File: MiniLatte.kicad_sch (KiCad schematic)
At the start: 23 parts, among them CN5 WAFER-PH2.0-4PZZ, CN6 47053-1000, CN8 SMTWE2055MTJ, CN9 SMTWE2055MTJ, SW6 DSHP01TSGER, U19 TPS54202DDCR, U22 W25N01GVZEIG_C907680

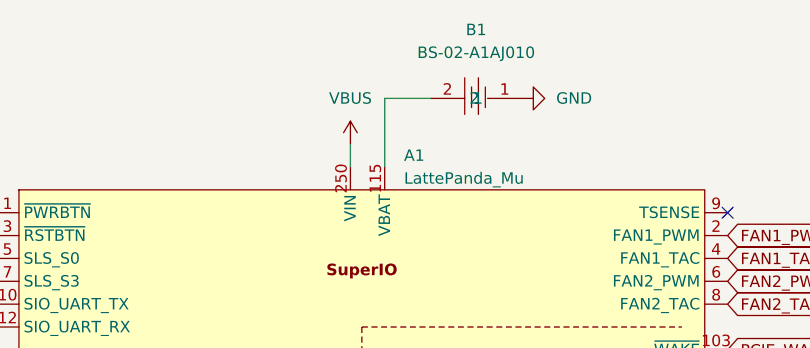
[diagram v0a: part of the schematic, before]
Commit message: .
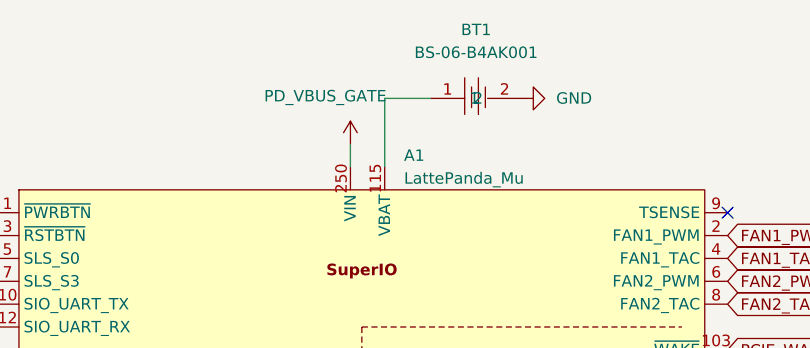
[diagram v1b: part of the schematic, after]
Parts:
- removed B1: BS-02-A1AJ010, easyeda2kicad:BAT-TH_BS-02-A1AJ010, symbol da:BS-02-A1AJ010
- added BT1: BS-06-B4AK001, easyeda2kicad:BAT-SMD_BS-06-B4AA012, symbol da:BS-06-B4AK001
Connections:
- net VBUS is gone; now on net PD_VBUS_GATE: A1.250 (VIN), A1.251 (VIN), A1.252 (VIN), A1.253 (VIN), A1.254 (VIN), A1.255 (VIN), A1.256 (VIN), A1.257 (VIN), A1.258 (VIN), A1.259 (VIN), A1.260 (VIN)
- net GND: now also BT1.2
- net at A1.115 (VBAT): now also BT1.1
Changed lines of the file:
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@@
-	)
-	(symbol
-		(lib_id "da:BS-02-A1AJ010")
-		(at 148.59 25.4 180)
-		(unit 1)
-		(exclude_from_sim no)
-		(in_bom yes)
-		(on_board yes)
-		(dnp no)
-		(fields_autoplaced yes)
-		(property "Reference" "B1"
-			(at 148.59 17.78 0)
-			(effects
-				(font
-					(size 1.27 1.27)
-				)
-			)
-		)
-		(property "Value" "BS-02-A1AJ010"
-			(at 148.59 20.32 0)
-			(effects
-				(font
-					(size 1.27 1.27)
-				)
-			)
-		)
-		(property "Footprint" "easyeda2kicad:BAT-TH_BS-02-A1AJ010"
-			(at 148.59 17.78 0)
-			(effects
-				(font
-					(size 1.27 1.27)
-				)
-				(hide yes)
-			)
-		)
-		(property "Datasheet" ""
-			(at 148.59 25.4 0)
-			(effects
-				(font
-					(size 1.27 1.27)
-				)
-				(hide yes)
-			)
-		)
-		(property "Description" ""
-			(at 148.59 25.4 0)
-			(effects
-				(font
-					(size 1.27 1.27)
-				)
-				(hide yes)
-			)
-		)
-		(property "LCSC Part" "C5239862"
-			(at 148.59 15.24 0)
-			(effects
-				(font
-					(size 1.27 1.27)
-				)
-				(hide yes)
-			)
-		)
-		(pin "1"
-		)
-		(pin "2"
-		)
-		(instances
-			(project ""
-				(path "/ffe475c5-d6e9-41b5-8ca1-322659dd88d8"
-					(reference "B1")
-					(unit 1)
-				)
-			)
-		)
 	)
 	(symbol
@@
 		(on_board yes)
 		(dnp no)
-		(fields_autoplaced yes)
 		(property "Reference" "#PWR04"
 			(at 134.62 34.29 0)
@@
 			)
 		)
-		(property "Value" "VBUS"
-			(at 134.62 25.4 0)
+		(property "Value" "PD_VBUS_GATE"
+			(at 131.826 25.146 0)
 			(effects
 				(font
@@
 					(unit 1)
 				)
+			)
+		)
+	)
+	(symbol
+		(lib_id "da:BS-06-B4AK001")
+		(at 148.59 25.4 0)
+		(unit 1)
+		(exclude_from_sim no)
+		(in_bom yes)
+		(on_board yes)
+		(dnp no)
+		(fields_autoplaced yes)
+		(property "Reference" "BT1"
+			(at 148.59 17.78 0)
+			(effects
+				(font
+					(size 1.27 1.27)
+				)
+			)
+		)
+		(property "Value" "BS-06-B4AK001"
+			(at 148.59 20.32 0)
+			(effects
+				(font
+					(size 1.27 1.27)
+				)
+			)
+		)
+		(property "Footprint" "easyeda2kicad:BAT-SMD_BS-06-B4AA012"
+			(at 148.59 33.02 0)
+			(effects
+				(font
+					(size 1.27 1.27)
+				)
+				(hide yes)
+			)
+		)
+		(property "Datasheet" ""
+			(at 148.59 25.4 0)
+			(effects
+				(font
+					(size 1.27 1.27)
+				)
+				(hide yes)
+			)
+		)
+		(property "Description" ""
+			(at 148.59 25.4 0)
+			(effects
+				(font
+					(size 1.27 1.27)
+				)
+				(hide yes)
+			)
+		)
+		(property "LCSC Part" "C964760"
+			(at 148.59 35.56 0)
+			(effects
+				(font
+					(size 1.27 1.27)
+				)
+				(hide yes)
+			)
+		)
+		(pin "2"
+		)
+		(pin "1"
+		)
+		(instances
+			(project ""
+				(path "/ffe475c5-d6e9-41b5-8ca1-322659dd88d8"
+					(reference "BT1")
+					(unit 1)
+				)

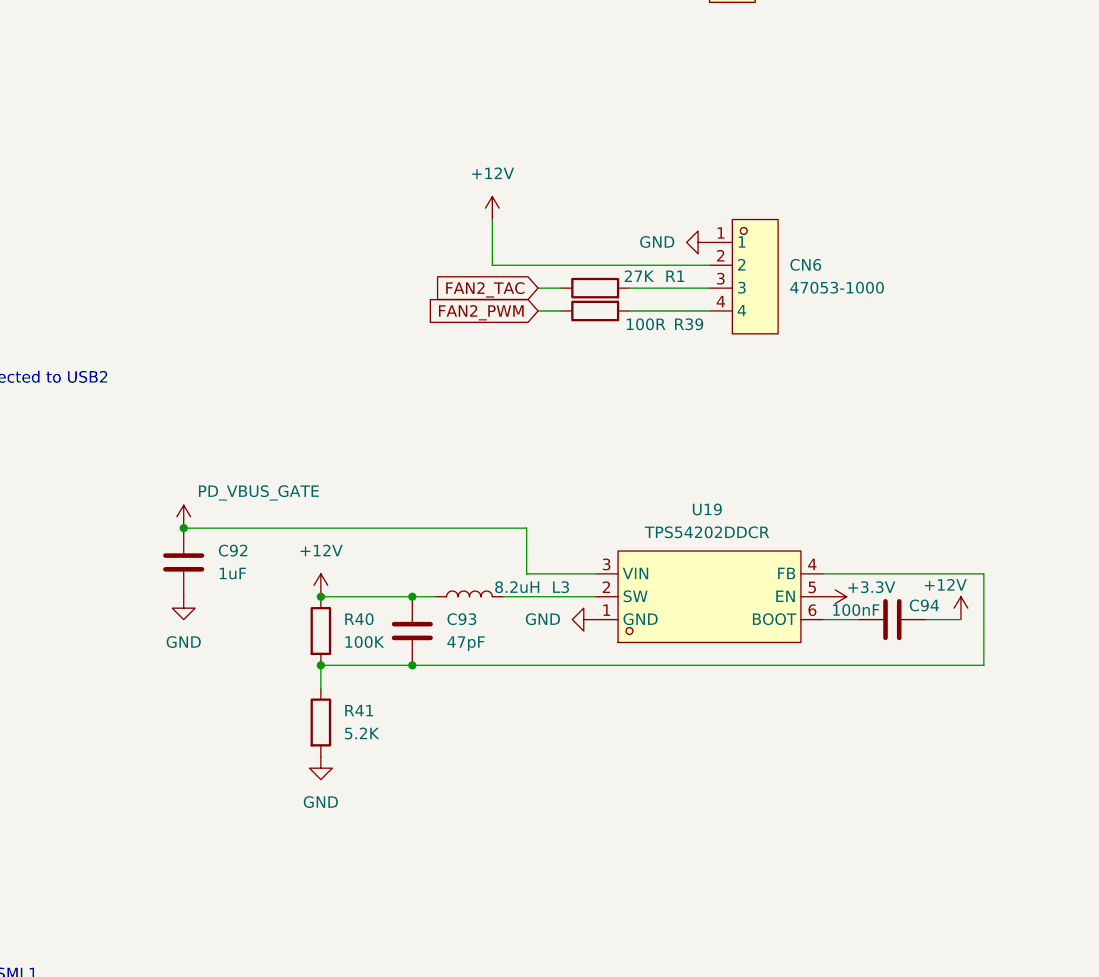
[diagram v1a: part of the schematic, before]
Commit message: .
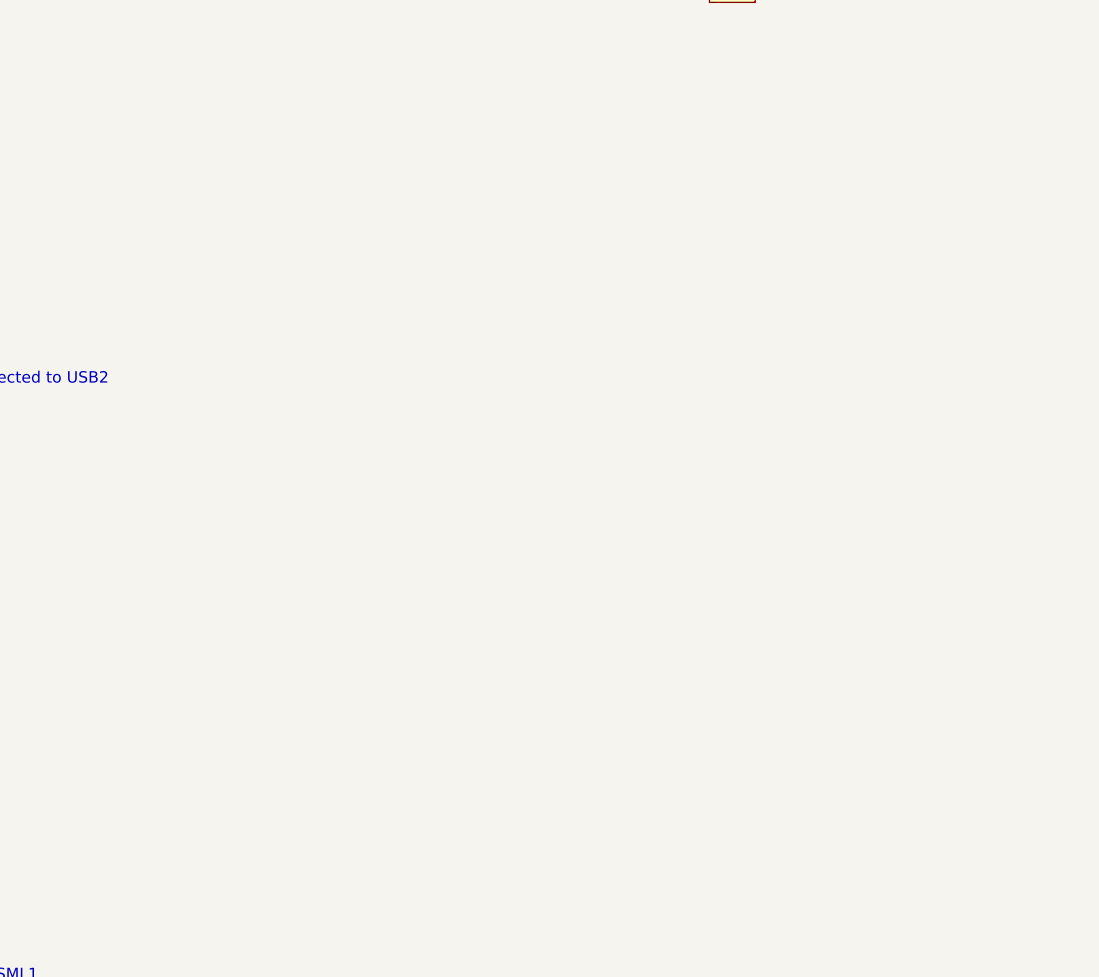
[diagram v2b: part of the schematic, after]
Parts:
- removed C92: 1uF, Capacitor_SMD:C_0603_1608Metric, symbol Device:C
- removed C93: 47pF, Capacitor_SMD:C_0402_1005Metric, symbol Device:C
- removed C94: 100nF, Capacitor_SMD:C_0402_1005Metric, symbol Device:C
- removed CN6: 47053-1000, easyeda2kicad:CONN-TH_47053-1000, symbol da:47053-1000
- removed L3: 8.2uH, Inductor_SMD:L_Changjiang_FXL0420, symbol Device:L
- removed R1: 27K, Resistor_SMD:R_0402_1005Metric, symbol Device:R
- removed R39: 100R, Resistor_SMD:R_0402_1005Metric, symbol Device:R
- removed R40: 100K, Resistor_SMD:R_0402_1005Metric, symbol Device:R
- removed R41: 5.2K, Resistor_SMD:R_0402_1005Metric, symbol Device:R
- removed U19: TPS54202DDCR, easyeda2kicad:SOT-23-6_L2.9-W1.6-P0.95-LS2.8-BL, symbol da:TPS54202DDCR
